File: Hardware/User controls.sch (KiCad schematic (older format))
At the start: 9 parts

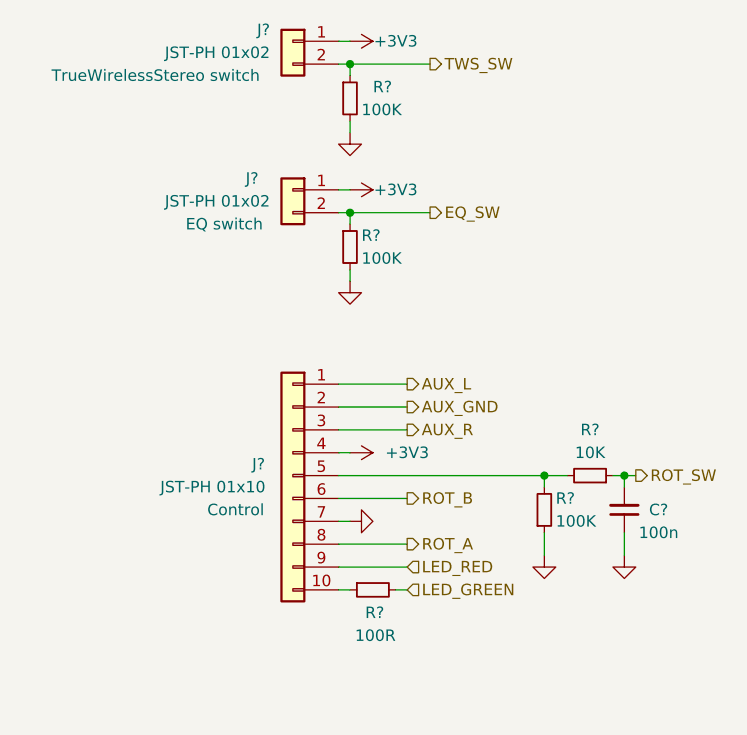
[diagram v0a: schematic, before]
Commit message: Pre refdes fix
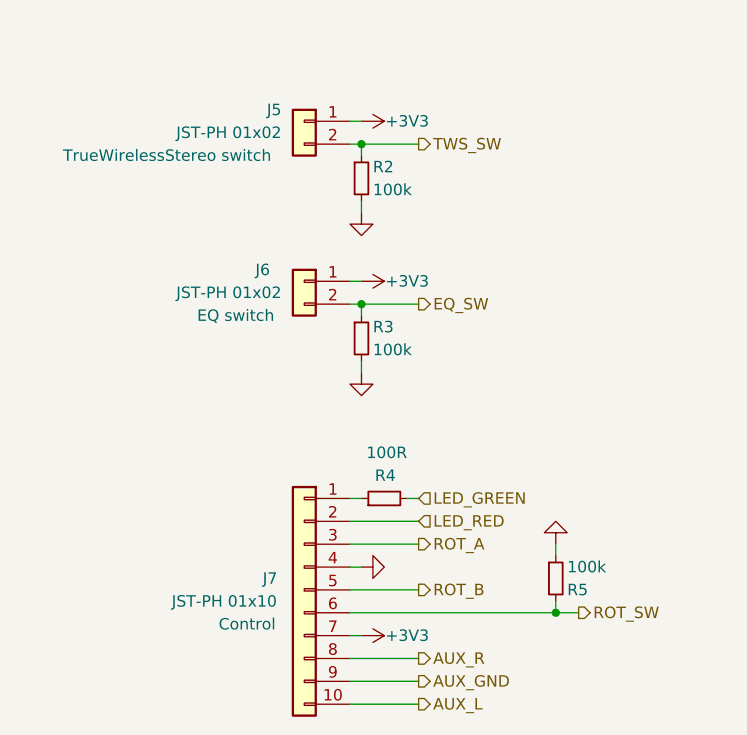
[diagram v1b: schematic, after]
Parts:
- removed C?: 100n, ZOUDIOfootprints:C0603, symbol Device:C_Small
- removed R?: 10K, ZOUDIOfootprints:R0603, symbol Device:R_Small
- J5, J6: renamed from J?; footprint ZOUDIOfootprints:JSTPH_2P -> Connector_JST:JST_PH_B2B-PH-K_1x02_P2.00mm_Vertical
- J7: renamed from J?; footprint ZOUDIOfootprints:JSTPH_10P -> Connector_JST:JST_PH_B10B-PH-K_1x10_P2.00mm_Vertical
- R2, R3, R5: renamed from R?; value 100K -> 100k; footprint ZOUDIOfootprints:R0603 -> Resistor_SMD:R_0603_1608Metric
- R4: renamed from R?; footprint ZOUDIOfootprints:R0603 -> Resistor_SMD:R_0603_1608Metric
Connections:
- net +3V3: now also J7.7 (Pin_7); no longer J7.4 (Pin_4)
- net AUX_GND: now also J7.9 (Pin_9); no longer J7.2 (Pin_2)
- net AUX_L: now also J7.10 (Pin_10); no longer J7.1 (Pin_1)
- net AUX_R: now also J7.8 (Pin_8); no longer J7.3 (Pin_3)
- net GND: now also J7.4 (Pin_4); no longer J7.7 (Pin_7)
- net LED_RED: now also J7.2 (Pin_2); no longer J7.9 (Pin_9)
- net ROT_A: now also J7.3 (Pin_3); no longer J7.8 (Pin_8)
- net ROT_B: now also J7.5 (Pin_5); no longer J7.6 (Pin_6)
- net ROT_SW: now also J7.6 (Pin_6), R5.2
- net at R4.1: now also J7.1 (Pin_1); no longer J7.10 (Pin_10)
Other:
- moved on the sheet: J5, J6, J7, R2, R3, R4, R5
